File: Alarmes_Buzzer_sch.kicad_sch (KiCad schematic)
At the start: 30 parts, among them Q58 2N7000, Q59 2N7000, Q60 2N7000, Q61 2N7000, Q62 2N7000, Q63 2N7000

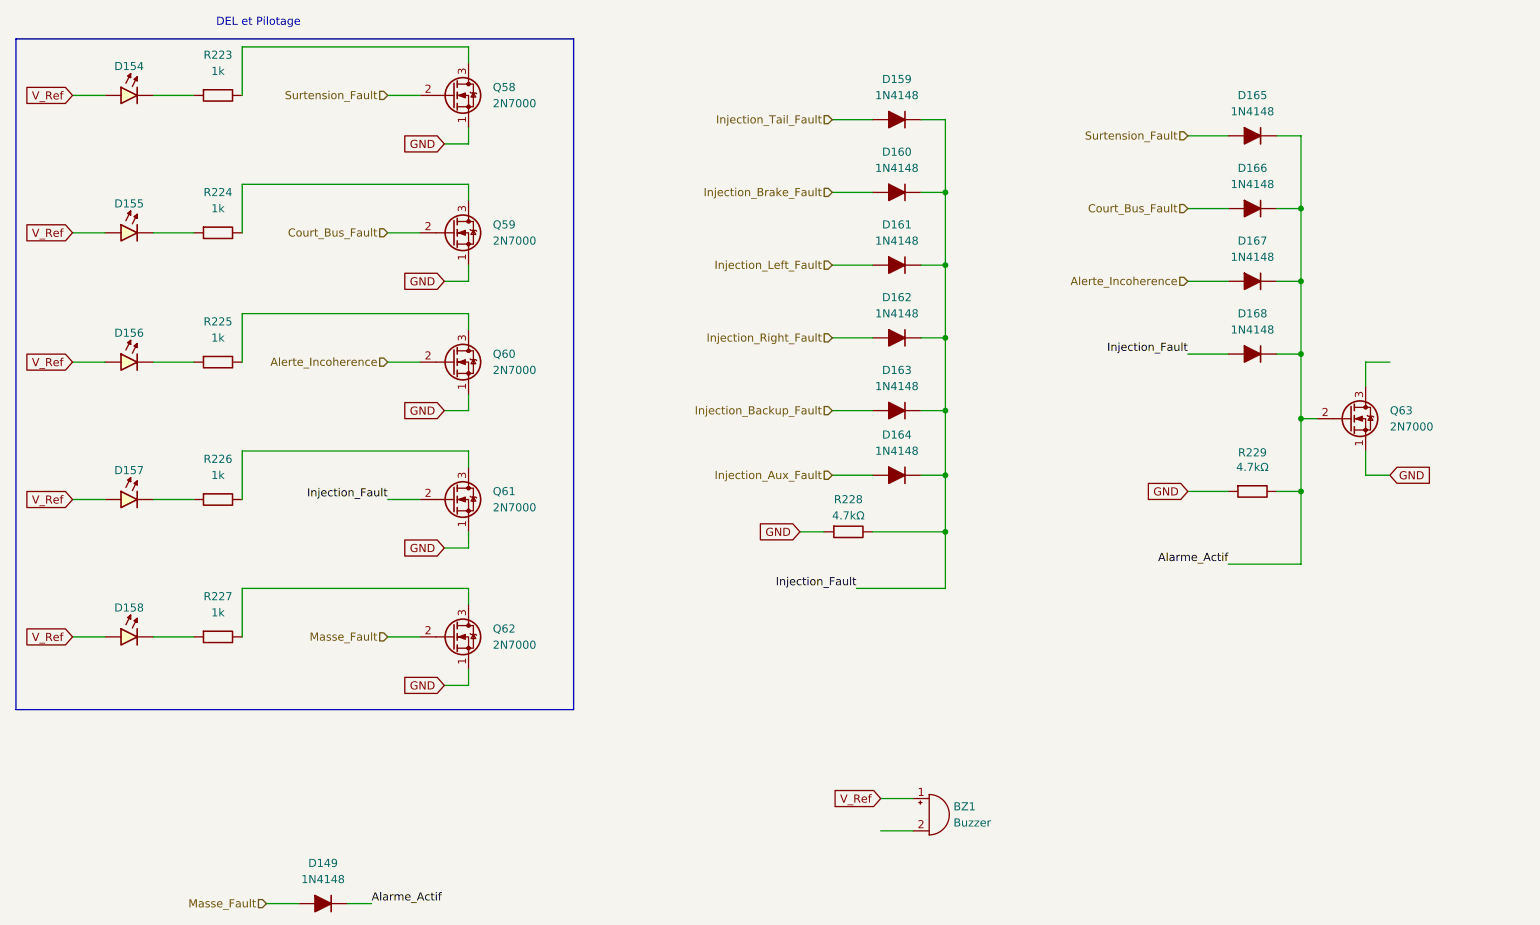
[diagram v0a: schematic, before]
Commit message: Add files via upload
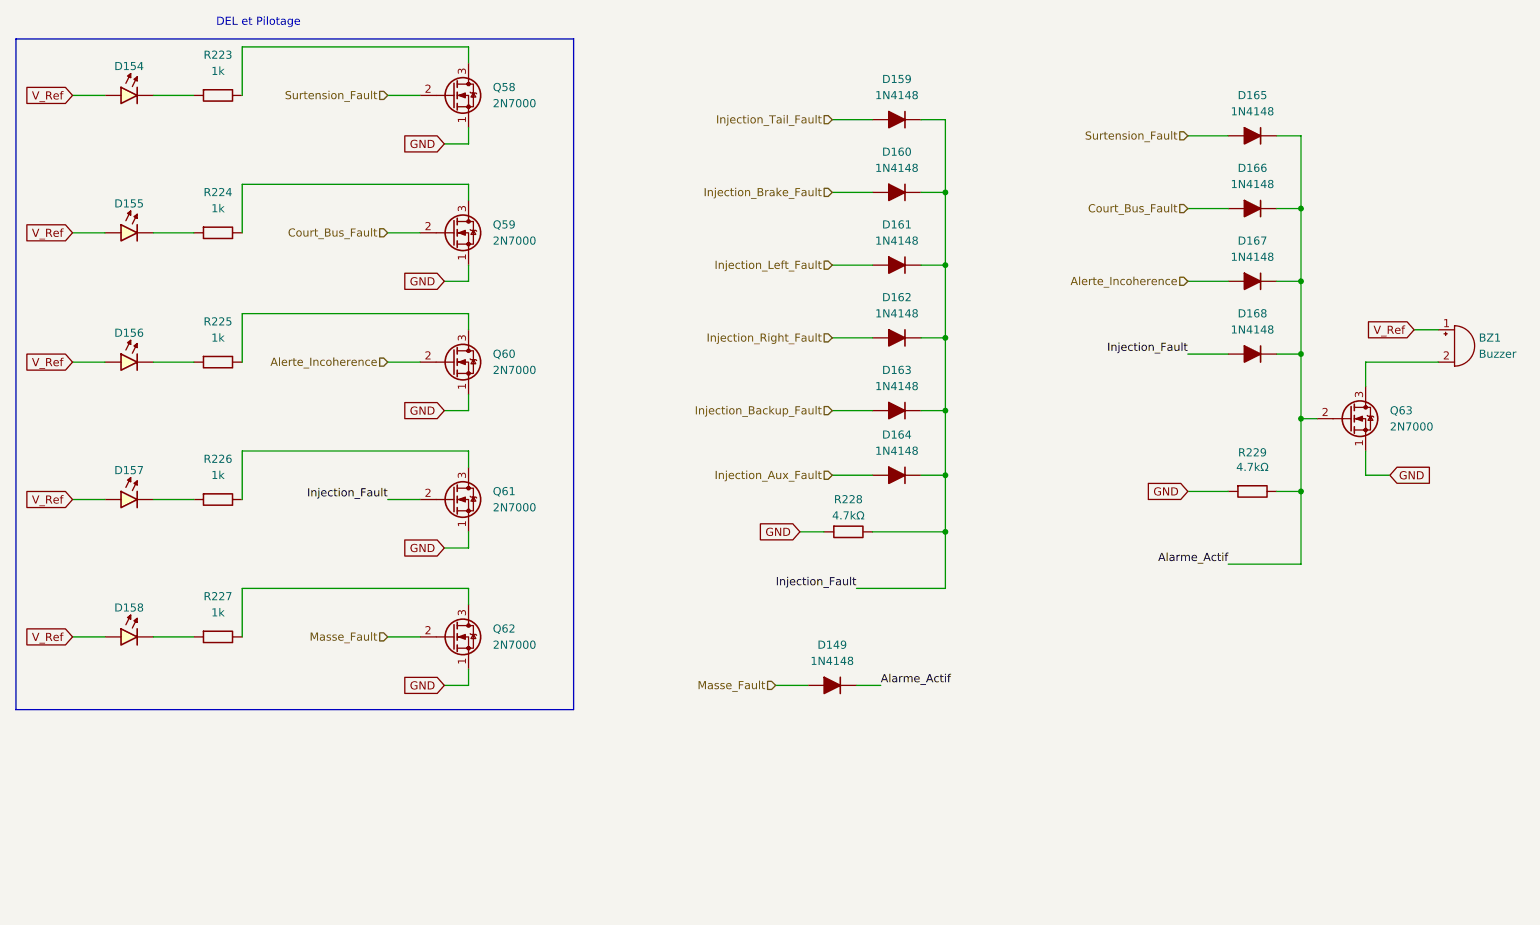
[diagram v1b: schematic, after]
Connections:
- net at Q63.3 (D): now also BZ1.2 (-)
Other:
- moved on the sheet: BZ1, D149
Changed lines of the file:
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@@
 	(wire
 		(pts
-			(xy 241.3 151.13) (xy 246.38 151.13)
-		)
-		(stroke
-			(width 0)
-			(type default)
-		)
-	)
-	(wire
-		(pts
 			(xy 127 77.47) (xy 133.35 77.47)
 		)
@@
 	(wire
 		(pts
-			(xy 241.3 146.05) (xy 246.38 146.05)
+			(xy 325.12 72.39) (xy 328.93 72.39)
 		)
 		(stroke
@@
 	(wire
 		(pts
-			(xy 317.5 77.47) (xy 321.31 77.47)
+			(xy 317.5 77.47) (xy 328.93 77.47)
 		)
 		(stroke
@@
 	(wire
 		(pts
-			(xy 157.48 162.56) (xy 161.29 162.56)
+			(xy 237.49 128.27) (xy 241.3 128.27)
 		)
 		(stroke
@@
 	(wire
 		(pts
-			(xy 144.78 162.56) (xy 149.86 162.56)
+			(xy 224.79 128.27) (xy 229.87 128.27)
 		)
 		(stroke
@@
 	)
 	(label "Alarme_Actif"
-		(at 161.29 162.56 0)
+		(at 241.3 128.27 0)
 		(effects
 			(font
@@
 	(global_label "V_Ref"
 		(shape input)
-		(at 241.3 146.05 180)
+		(at 325.12 72.39 180)
 		(fields_autoplaced yes)
 		(effects
@@
 		)
 		(property "Intersheetrefs" "${INTERSHEET_REFS}"
-			(at 233.1743 146.05 0)
+			(at 316.9943 72.39 0)
 			(hide yes)
 			(show_name no)
@@
 	(hierarchical_label "Masse_Fault"
 		(shape input)
-		(at 144.78 162.56 180)
+		(at 224.79 128.27 180)
 		(effects
 			(font
@@
 	(symbol
 		(lib_id "Device:Buzzer")
-		(at 248.92 148.59 0)
+		(at 331.47 74.93 0)
 		(unit 1)
 		(body_style 1)
@@
 		(fields_autoplaced yes)
 		(property "Reference" "BZ1"
-			(at 252.73 147.3199 0)
+			(at 335.28 73.6599 0)
 			(show_name no)
 			(do_not_autoplace no)
@@
 		)
 		(property "Value" "Buzzer"
-			(at 252.73 149.8599 0)
+			(at 335.28 76.1999 0)
 			(show_name no)
 			(do_not_autoplace no)
@@
 		)
 		(property "Footprint" ""
-			(at 248.285 146.05 90)
+			(at 330.835 72.39 90)
 			(hide yes)
 			(show_name no)
@@
 		)
 		(property "Datasheet" ""
-			(at 248.285 146.05 90)
+			(at 330.835 72.39 90)
 			(hide yes)
 			(show_name no)
@@
 		)
 		(property "Description" "Buzzer, polarized"
-			(at 248.92 148.59 0)
+			(at 331.47 74.93 0)
 			(hide yes)
 			(show_name no)
@@
 	(symbol
 		(lib_id "PCM_Diode_AKL:1N4148")
-		(at 153.67 162.56 0)
+		(at 233.68 128.27 0)
 		(unit 1)
 		(body_style 1)
@@
 		(fields_autoplaced yes)
 		(property "Reference" "D149"
-			(at 153.67 156.21 0)
+			(at 233.68 121.92 0)
 			(show_name no)
 			(do_not_autoplace no)
@@
 		)
 		(property "Value" "1N4148"
-			(at 153.67 158.75 0)
+			(at 233.68 124.46 0)
 			(show_name no)
 			(do_not_autoplace no)
@@
 		)
 		(property "Footprint" "PCM_Diode_THT_AKL:D_DO-35_SOD27_P7.62mm_Horizontal"
-			(at 153.67 162.56 0)
+			(at 233.68 128.27 0)
 			(hide yes)
 			(show_name no)
@@
 		)
 		(property "Datasheet" "https://datasheet.octopart.com/1N4148TR-ON-Semiconductor-datasheet-42765246.pdf"
-			(at 153.67 162.56 0)
+			(at 233.68 128.27 0)
 			(hide yes)
 			(show_name no)
@@
 		)
 		(property "Description" "DO-35 Diode, Small Signal, Fast Switching, 75V, 150mA, 4ns, Alternate KiCad Library"
-			(at 153.67 162.56 0)
+			(at 233.68 128.27 0)
 			(hide yes)
 			(show_name no)

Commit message: Add files via upload
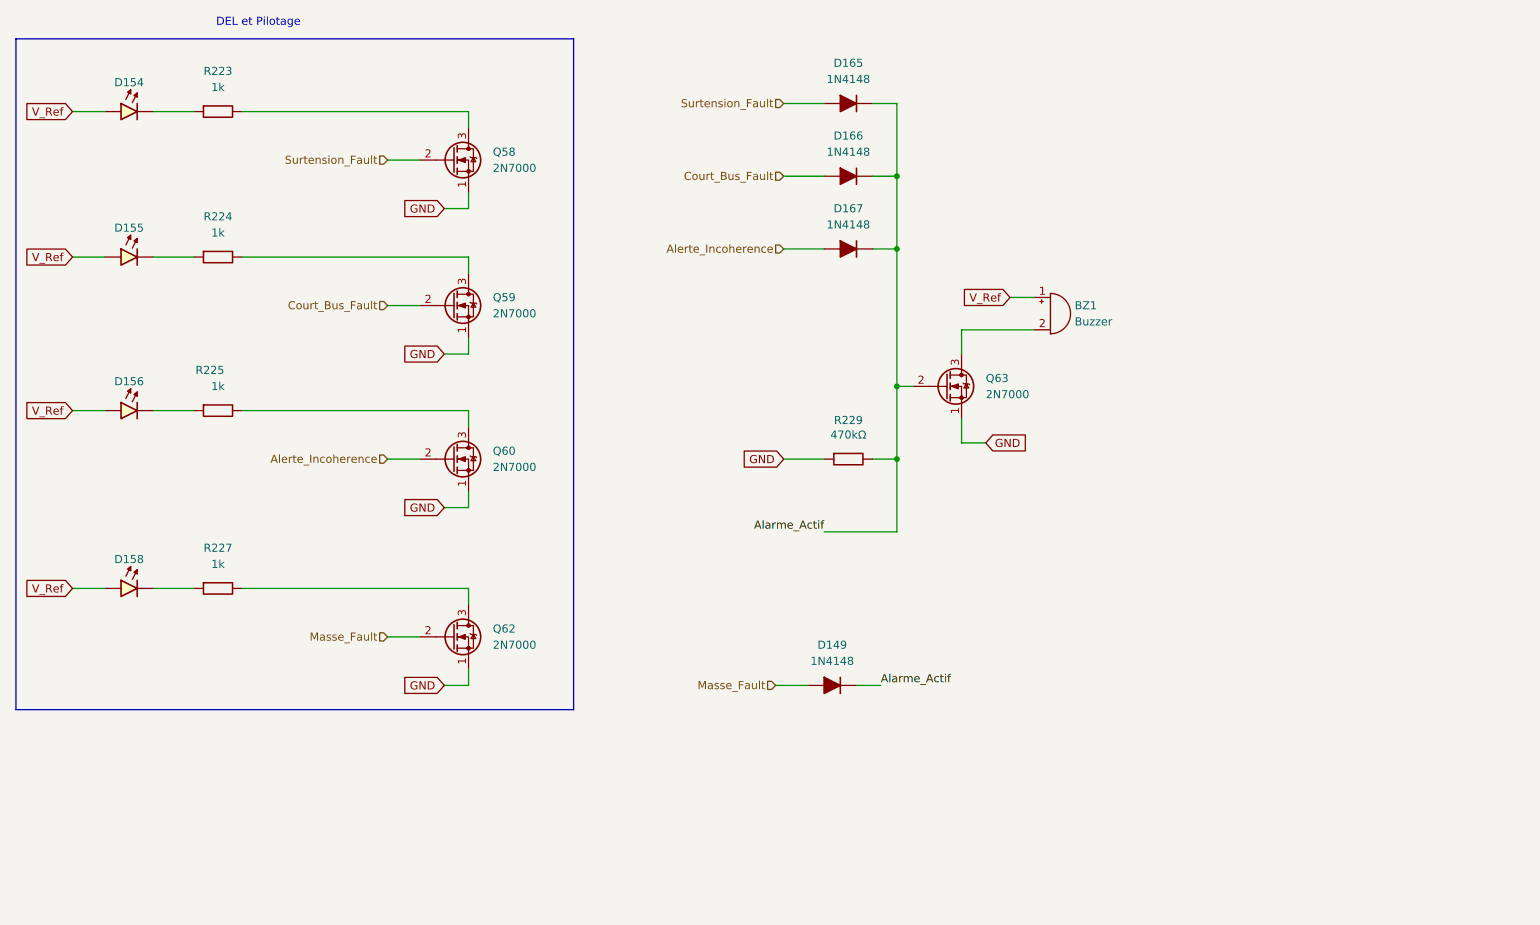
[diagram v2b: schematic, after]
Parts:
- removed D157: LED_2x5mm_Horizontal_Red, PCM_LED_THT_AKL:LED_Rectangular_W5.0mm_H2.0mm_Horizontal_O3.81mm_Z1.0mm, symbol PCM_LED_AKL:LED_2x5mm_Horizontal_Red
- removed D159, D160, D161, D162, D163, D164, D168: 1N4148, PCM_Diode_THT_AKL:D_DO-35_SOD27_P7.62mm_Horizontal, symbol PCM_Diode_AKL:1N4148
- removed Q61: 2N7000, Package_TO_SOT_THT:TO-92_Inline, symbol Transistor_FET:2N7000
- removed R226: 1k, Resistor_THT:R_Axial_DIN0207_L6.3mm_D2.5mm_P10.16mm_Horizontal, symbol PCM_SL_Resistors:1k
- removed R228: 4.7kΩ, Resistor_THT:R_Axial_DIN0207_L6.3mm_D2.5mm_P10.16mm_Horizontal, symbol PCM_SL_Resistors:1k
- R229: value 4.7kΩ -> 470kΩ
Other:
- moved on the sheet: BZ1, D154, D155, D156, D158, D165, D166, D167, Q58, Q59, Q60, Q63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
